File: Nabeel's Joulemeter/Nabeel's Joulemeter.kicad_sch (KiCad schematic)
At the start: 50 parts, among them J1 XT60-M, J2 XT60-M, J3 22035035, J4 22035035, U1 INA181A1QDBVRQ1, U2 PADS131M04QPWRQ1, U3 UA78M05QDCYRG4Q1, U4 MCP6286T-E/OT

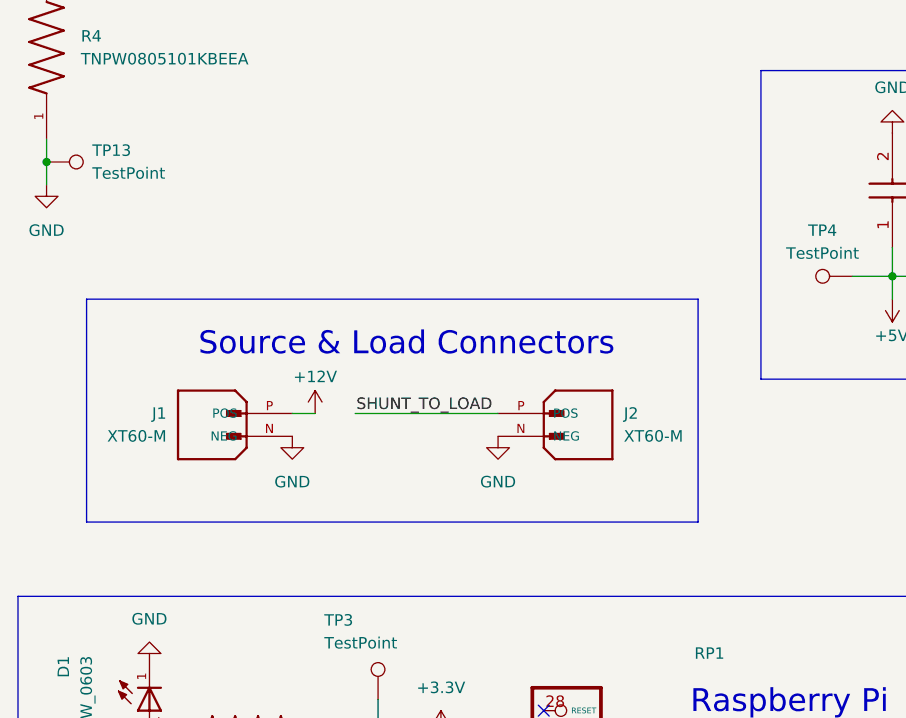
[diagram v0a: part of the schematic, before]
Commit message: latest schematic and pcb draft
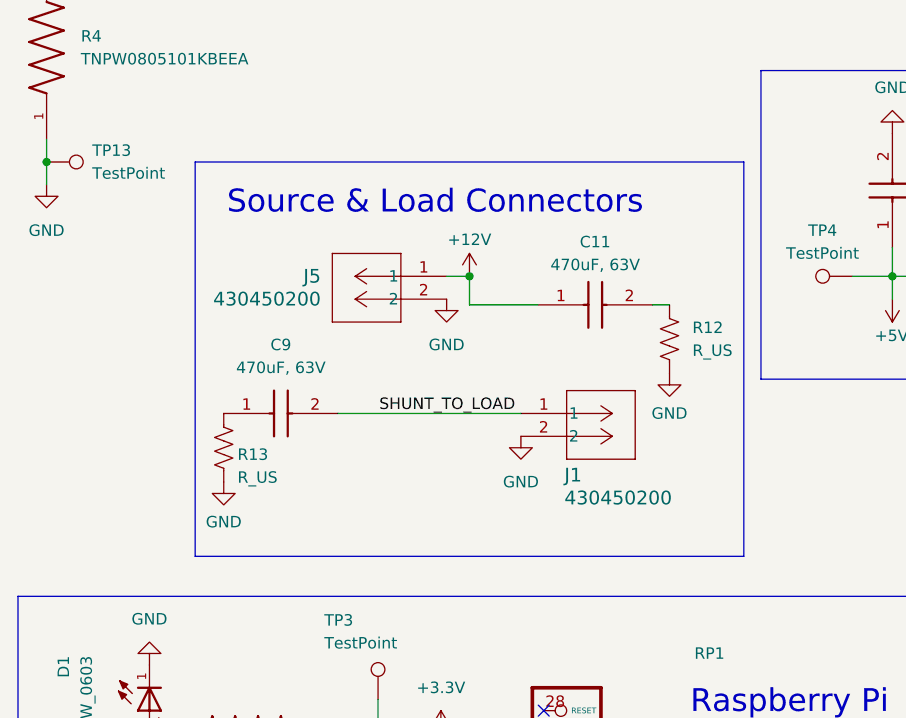
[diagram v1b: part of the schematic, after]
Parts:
- removed J1, J2: XT60-M, SMV_Connectors:AMASS_XT60-M, symbol SMV_Custom:XT60-M
- added C11, C9: 470uF, 63V, SMV_Passives:Big_Chunky_Cap, symbol SMV_Custom:Big_Chunky_Cap2
- added J1, J5: 430450200, SMV_Connectors:CONN_SD-43045-001_02_MOL, symbol SMV_Custom:430450200
- added R12, R13: R_US, Resistor_THT:R_Axial_DIN0204_L3.6mm_D1.6mm_P1.90mm_Vertical, symbol Device:R_US
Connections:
- net +12V: now also C11.1, J5.1
- net GND: now also J1.2, J5.2, R12.2, R13.2
- net SHUNT_TO_LOAD: now also C9.2, J1.1
- new net: C11.2, R12.1
- new net: C9.1, R13.1
